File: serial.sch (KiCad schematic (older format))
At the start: 8 parts, among them J18 DE9 Male (RS-232), U8 MAX232

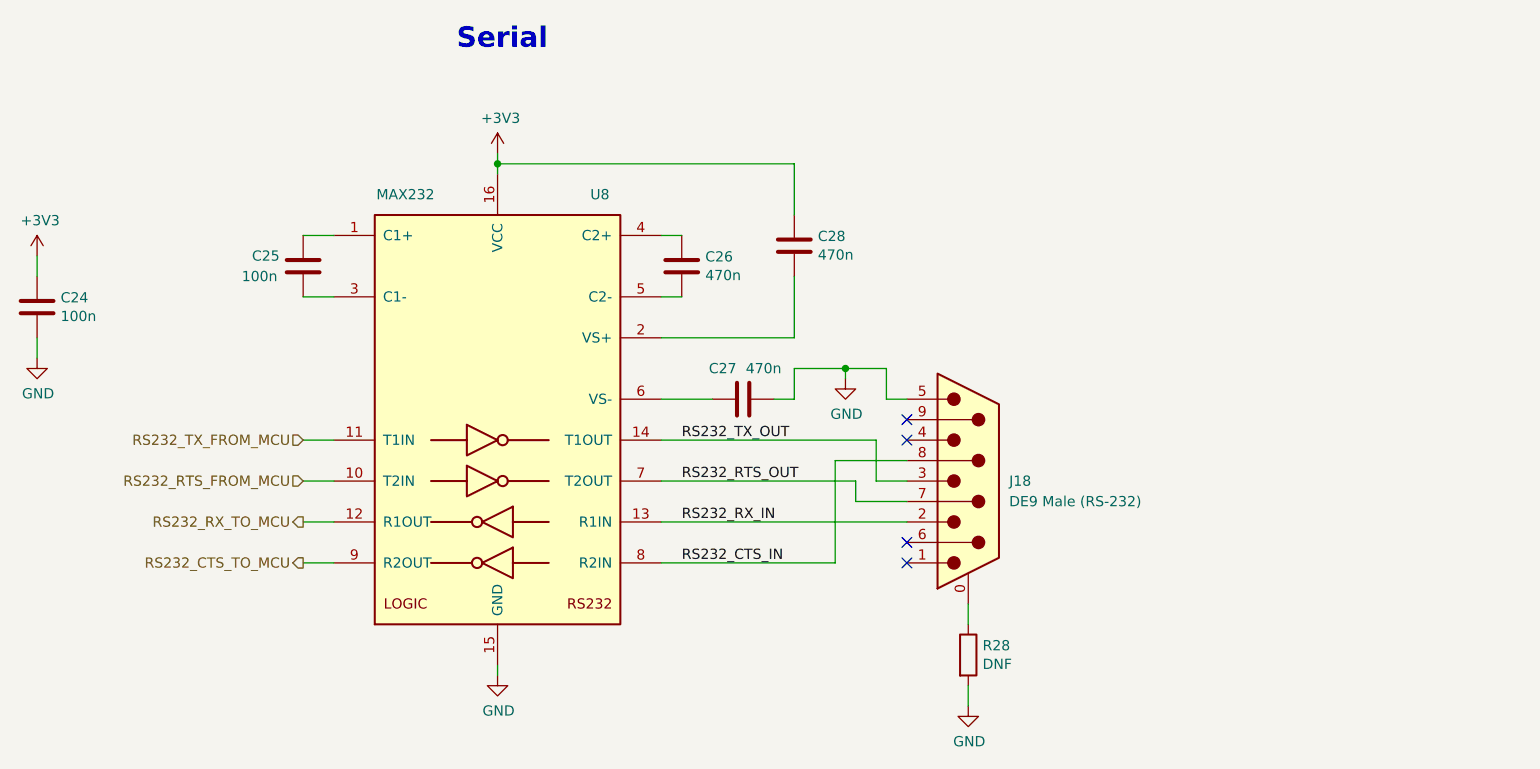
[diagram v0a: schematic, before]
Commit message: Work in progress.
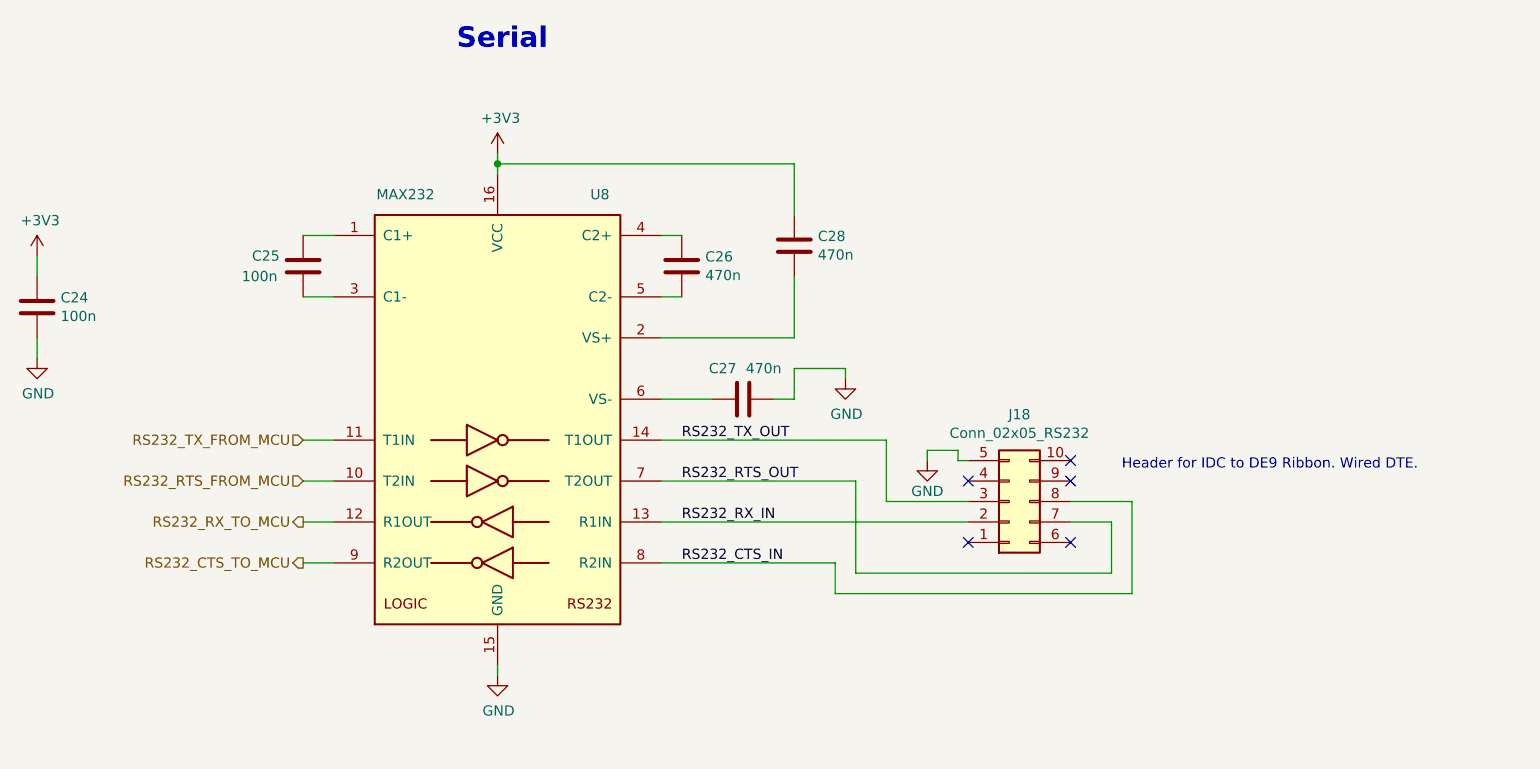
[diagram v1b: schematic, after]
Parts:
- removed J18: DE9 Male (RS-232), Connector_Dsub:DSUB-9_Male_Horizontal_P2.77x2.84mm_EdgePinOffset4.94mm_Housed_MountingHolesOffset7.48mm, symbol Connector:DB9_Male_MountingHoles
- removed R28: DNF, Resistor_THT:R_Axial_DIN0411_L9.9mm_D3.6mm_P12.70mm_Horizontal, symbol Device:R
- added J18: Conn_02x05_RS232, Connector_PinHeader_2.54mm:PinHeader_2x05_P2.54mm_Vertical, symbol Connector_Generic:Conn_02x05_Top_Bottom
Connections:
- net GND: now also J18.5 (Pin_5)
- net RS232_CTS_IN: now also J18.8 (Pin_8)
- net RS232_RTS_OUT: now also J18.7 (Pin_7)
- net RS232_RX_IN: now also J18.2 (Pin_2)
- net RS232_TX_OUT: now also J18.3 (Pin_3)
- no-connect marks 4 -> 5
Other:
- note added: "Header for IDC to DE9 Ribbon. Wired DTE."
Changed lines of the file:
@@
 Comment4 ""
 $EndDescr
-$Comp
-L Connector:DB9_Male_MountingHoles J?
-U 1 1 5DF3B98B
-P 7900 3950
-AR Path="/5DF3B98B" Ref="J?"  Part="1"
-AR Path="/5DF2601D/5DF3B98B" Ref="J18"  Part="1"
-F 0 "J18" H 8100 3950 50  0000 L CNN
-F 1 "DE9 Male (RS-232)" H 8100 3850 50  0000 L CNN
-F 2 "Connector_Dsub:DSUB-9_Male_Horizontal_P2.77x2.84mm_EdgePinOffset4.94mm_Housed_MountingHolesOffset7.48mm" H 7900 3950 50  0001 C CNN
-F 3 " ~" H 7900 3950 50  0001 C CNN
-	1    7900 3950
-	1    0    0    -1
-$EndComp
 Text HLabel 4650 3750 0    50   Input ~ 0
 RS232_TX_FROM_MCU
@@
 Wire Wire Line
 	4650 4350 4800 4350
-NoConn ~ 7600 3650
-NoConn ~ 7600 3750
-NoConn ~ 7600 4250
-NoConn ~ 7600 4350
-Wire Wire Line
-	7600 3950 7450 3950
-Wire Wire Line
-	7450 3750 6400 3750
-Wire Wire Line
-	7450 3750 7450 3950
-Wire Wire Line
-	7600 4150 6400 4150
 Text Label 6500 4350 0    50   ~ 0
 RS232_CTS_IN
@@
 Text Label 6500 3950 0    50   ~ 0
 RS232_RTS_OUT
-Wire Wire Line
-	6400 3950 7350 3950
-Wire Wire Line
-	7350 4050 7350 3950
-Wire Wire Line
-	7350 4050 7600 4050
-Wire Wire Line
-	6400 4350 7250 4350
-Wire Wire Line
-	7250 3850 7600 3850
-Wire Wire Line
-	7250 3850 7250 4350
 $Comp
 L power:GND #PWR072
@@
 Wire Wire Line
 	7300 3450 7300 3400
-Wire Wire Line
-	7300 3400 7500 3400
-Wire Wire Line
-	7500 3400 7500 3550
-Wire Wire Line
-	7500 3550 7600 3550
-$Comp
-L Device:R R28
-U 1 1 5E180C9A
-P 7900 4800
-F 0 "R28" H 7970 4846 50  0000 L CNN
-F 1 "DNF" H 7970 4755 50  0000 L CNN
-F 2 "Resistor_THT:R_Axial_DIN0411_L9.9mm_D3.6mm_P12.70mm_Horizontal" V 7830 4800 50  0001 C CNN
-F 3 "~" H 7900 4800 50  0001 C CNN
-	1    7900 4800
-	1    0    0    -1
-$EndComp
-$Comp
-L power:GND #PWR073
-U 1 1 5E181402
-P 7900 5050
-F 0 "#PWR073" H 7900 4800 50  0001 C CNN
-F 1 "GND" H 7905 4877 50  0000 C CNN
-F 2 "" H 7900 5050 50  0001 C CNN
-F 3 "" H 7900 5050 50  0001 C CNN
-	1    7900 5050
-	1    0    0    -1
-$EndComp
-Wire Wire Line
-	7900 5050 7900 4950
-Wire Wire Line
-	7900 4650 7900 4550
 $Comp
 L Device:C C26
@@
 Wire Wire Line
 	7050 3400 7300 3400
-Connection ~ 7300 3400
 Wire Wire Line
 	5600 2400 7050 2400
@@
 Text Notes 5400 1850 0    100  ~ 20
 Serial
+NoConn ~ 8400 3850
+NoConn ~ 7900 4250
+NoConn ~ 8400 4250
+NoConn ~ 7900 3950
+NoConn ~ 8400 3950
+$Comp
+L Connector_Generic:Conn_02x05_Top_Bottom J18
+U 1 1 5E02DBC9
+P 8100 4050
+F 0 "J18" H 8150 3625 50  0000 C CNN
+F 1 "Conn_02x05_RS232" H 8150 3716 50  0000 C CNN
+F 2 "Connector_PinHeader_2.54mm:PinHeader_2x05_P2.54mm_Vertical" H 8100 4050 50  0001 C CNN
+F 3 "~" H 8100 4050 50  0001 C CNN
+	1    8100 4050
+	1    0    0    1
+$EndComp
+$Comp
+L power:GND #PWR0101
+U 1 1 5E03D39E
+P 7700 3850
+F 0 "#PWR0101" H 7700 3600 50  0001 C CNN
+F 1 "GND" H 7700 3700 50  0000 C CNN
+F 2 "" H 7700 3850 50  0001 C CNN
+F 3 "" H 7700 3850 50  0001 C CNN
+	1    7700 3850
+	1    0    0    -1
+$EndComp
+Wire Wire Line
+	7700 3850 7700 3800
+Wire Wire Line
+	7700 3800 7850 3800
+Wire Wire Line
+	7850 3800 7850 3850
+Wire Wire Line
+	7850 3850 7900 3850
+Wire Wire Line
+	7500 3750 6400 3750
+Wire Wire Line
+	6400 4150 7900 4150
+Wire Wire Line
+	7900 4050 7500 4050
+Wire Wire Line
+	7500 3750 7500 4050
+Wire Wire Line
+	6400 3950 7350 3950
+Wire Wire Line
+	8700 4050 8400 4050
+Wire Wire Line
+	8600 4150 8400 4150
+Wire Wire Line
+	7250 4350 7250 4500
+Wire Wire Line
+	6400 4350 7250 4350
+Wire Wire Line
+	8600 4150 8600 4400
+Wire Wire Line
+	7350 3950 7350 4400
+Wire Wire Line
+	7350 4400 8600 4400
+Wire Wire Line
+	7250 4500 8700 4500
+Wire Wire Line
+	8700 4050 8700 4500
+Text Notes 8650 3900 0    50   ~ 0
+Header for IDC to DE9 Ribbon. Wired DTE.
 $EndSCHEMATC
